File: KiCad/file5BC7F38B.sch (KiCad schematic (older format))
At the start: 54 parts, among them J307 Jumper_NC_Small, P301 ISP/PDI, P302 Thru, P303 Header, P304 Header, U301 DS3231, U302 TS5A3157, U303 ATMEGA328P, U304 SI5351A, U305 74HC1G08, U306 MIC5219-3.3BM5, U307 SN74CB3Q3305, U308 MIC5219-3.3BM5, X301 ASTX-H11-25.MHZ

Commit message: Changes for FlexFox80
Wholesale changes for new project.
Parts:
- removed C303: 100nF, Capacitors_SMD:C_0805_HandSoldering, symbol Device:C_Small
- removed U302: TS5A3157, TO_SOT_Packages_SMD:SOT-363_Handsolder, symbol ARDF-2-Band-MiniTx-rescue:TS5A3159
- added U?: ATmega1284P-AU, Package_QFP:TQFP-44_10x10mm_P0.8mm, symbol MCU_Microchip_ATmega:ATmega1284P-AU
- BT301: symbol ARDF-2-Band-MiniTx-rescue:Battery_Single_Cell -> FlexFox80-rescue:Battery_Single_Cell-ARDF-2-Band-MiniTx-rescue
- D301: symbol ARDF-2-Band-MiniTx-rescue:D_Schottky_x2_KCom_Dual -> FlexFox80-rescue:D_Schottky_x2_KCom_Dual-ARDF-2-Band-MiniTx-rescue
- D302: symbol ARDF-2-Band-MiniTx-rescue:ZENER -> FlexFox80-rescue:ZENER-ARDF-2-Band-MiniTx-rescue
- D303: symbol ARDF-2-Band-MiniTx-rescue:MBD54DWT1G_Schottky_Ind -> FlexFox80-rescue:MBD54DWT1G_Schottky_Ind-ARDF-2-Band-MiniTx-rescue
- P301: symbol ARDF-2-Band-MiniTx-rescue:CONN_02X03 -> FlexFox80-rescue:CONN_02X03-ARDF-2-Band-MiniTx-rescue
- P302, W307, W308: symbol ARDF-2-Band-MiniTx-rescue:CONN_01X01 -> FlexFox80-rescue:CONN_01X01-ARDF-2-Band-MiniTx-rescue
- P303, P304: symbol ARDF-2-Band-MiniTx-rescue:CONN_01X06 -> FlexFox80-rescue:CONN_01X06-ARDF-2-Band-MiniTx-rescue
- TP301: symbol ARDF-2-Band-MiniTx-rescue:CONN_01X03 -> FlexFox80-rescue:CONN_01X03-ARDF-2-Band-MiniTx-rescue
- U303: symbol ARDF-2-Band-MiniTx-rescue:ATMEGA328P-A -> FlexFox80-rescue:ATMEGA328P-A-ARDF-2-Band-MiniTx-rescue
- U305: symbol ARDF-2-Band-MiniTx-rescue:74HC1G08 -> FlexFox80-rescue:74HC1G08-ARDF-2-Band-MiniTx-rescue
- U306, U308: symbol ARDF-2-Band-MiniTx-rescue:MIC5219 -> FlexFox80-rescue:MIC5219-ARDF-2-Band-MiniTx-rescue
- U307: symbol ARDF-2-Band-MiniTx-rescue:SN74CB3Q3305 -> FlexFox80-rescue:SN74CB3Q3305-ARDF-2-Band-MiniTx-rescue
- W301, W302, W309, W310, W311, W312, W313, W314, W315, W316: symbol ARDF-2-Band-MiniTx-rescue:TEST_1P -> FlexFox80-rescue:TEST_1P-ARDF-2-Band-MiniTx-rescue
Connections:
- net labels removed: VHF_CLK
- wire segments 189 -> 245
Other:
- note added: "PCB: Flex Fox 80 ARDF Transmitter (p. 3/3)"
- note removed: "PCB: Dual-Band Transmitter (p. 3/3)"

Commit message: Schematic
Schematic changes for FlexFox80
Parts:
- removed U303: ATMEGA328P, Housings_QFP:TQFP-32_7x7mm_Pitch0.8mm, symbol FlexFox80-rescue:ATMEGA328P-A-ARDF-2-Band-MiniTx-rescue
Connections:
- net labels added: ADC3, ADC4, HT_AUDIO_IN, INT2, PC4, PC5, RXD0, RXD1, TXD0, TXD1
- net labels removed: 2M_ANTENNA_DETECT, PD2, VHF_ENABLE
- wire segments 245 -> 263
- no-connect marks 12 -> 24
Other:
- moved on the sheet: BT301, C301, C302, C304, C305, C306, C307, C308, C310, C312, C314, C316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

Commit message: Schematic Updates
More schematic changes
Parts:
- removed J307: Jumper_NC_Small, Wire_Connections_Bridges:Solder-Jumper-NC-SMD-Pad_Small, symbol Device:Jumper_NC_Small
- added Y301: 20 MHz, symbol Device:Resonator_Small
- gave numbers to parts that had none: 1
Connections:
- net labels added: KEY_OUT, PA0, PA1, PA2, PA3, PC6, PC7, PTT_OUT, TONE_OUT
- net labels removed: PB2, PB6, PB7, PC0, PC1, PD0, PD1, PD3, VHF_CLK_SEL
- wire segments 263 -> 258
- no-connect marks 24 -> 17
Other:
- moved on the sheet: C309, D303A, P303, R304, R305

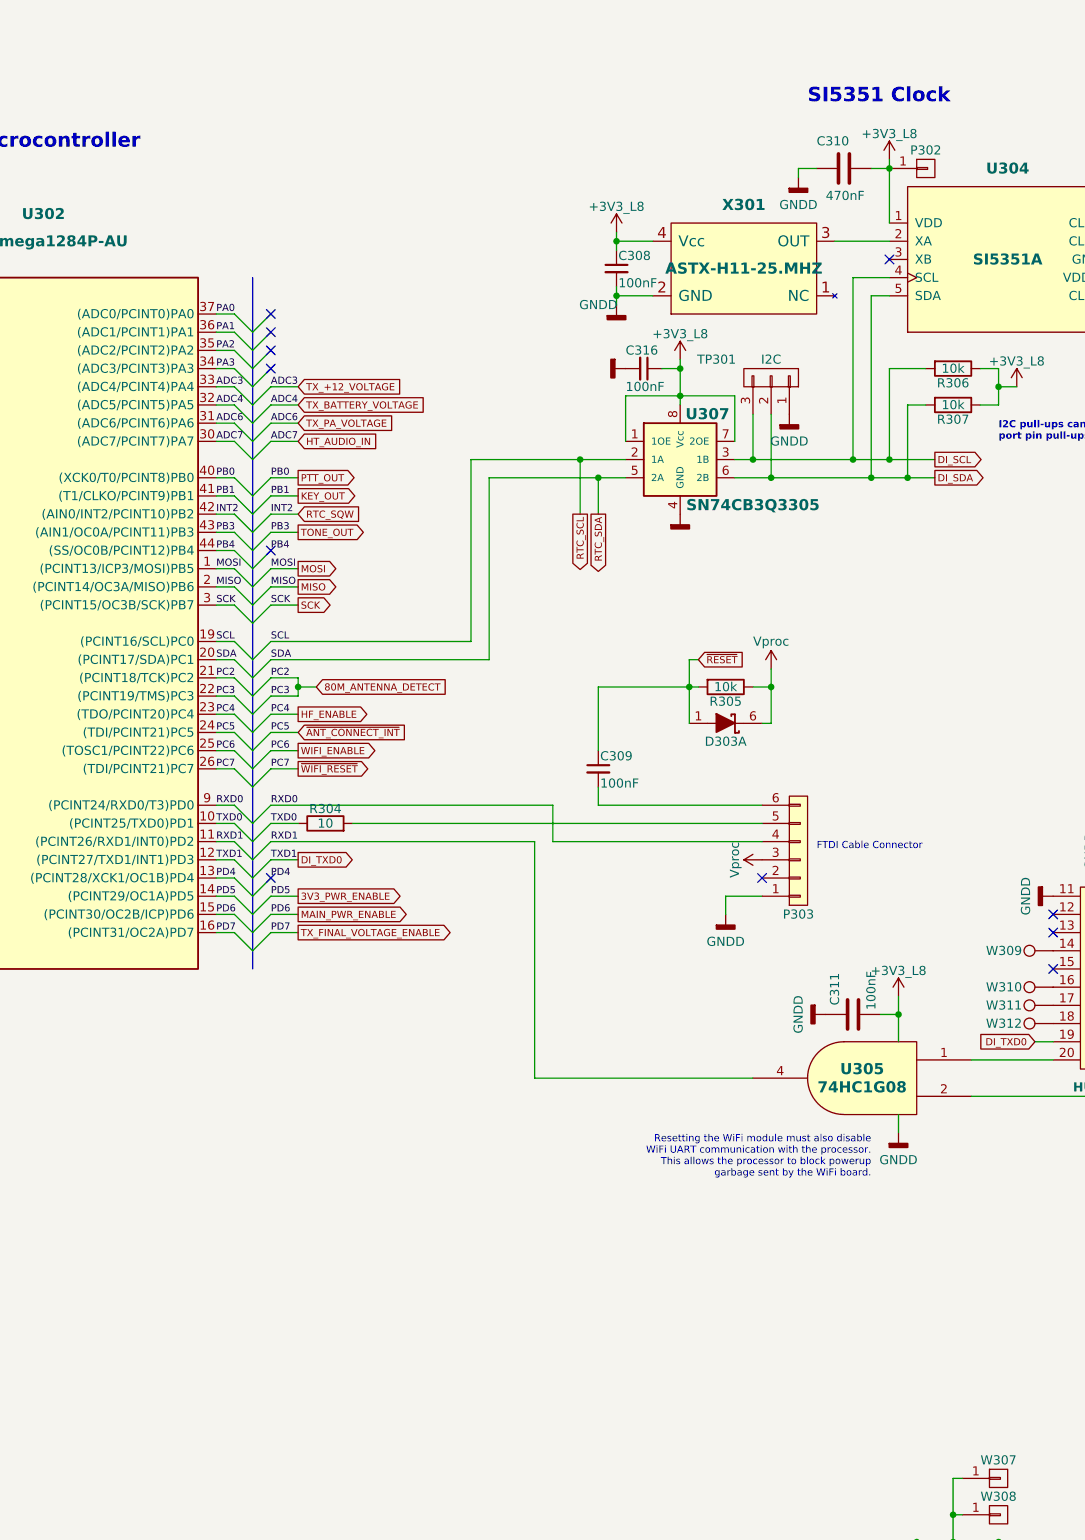
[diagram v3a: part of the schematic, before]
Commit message: Schematic changes
Schematic
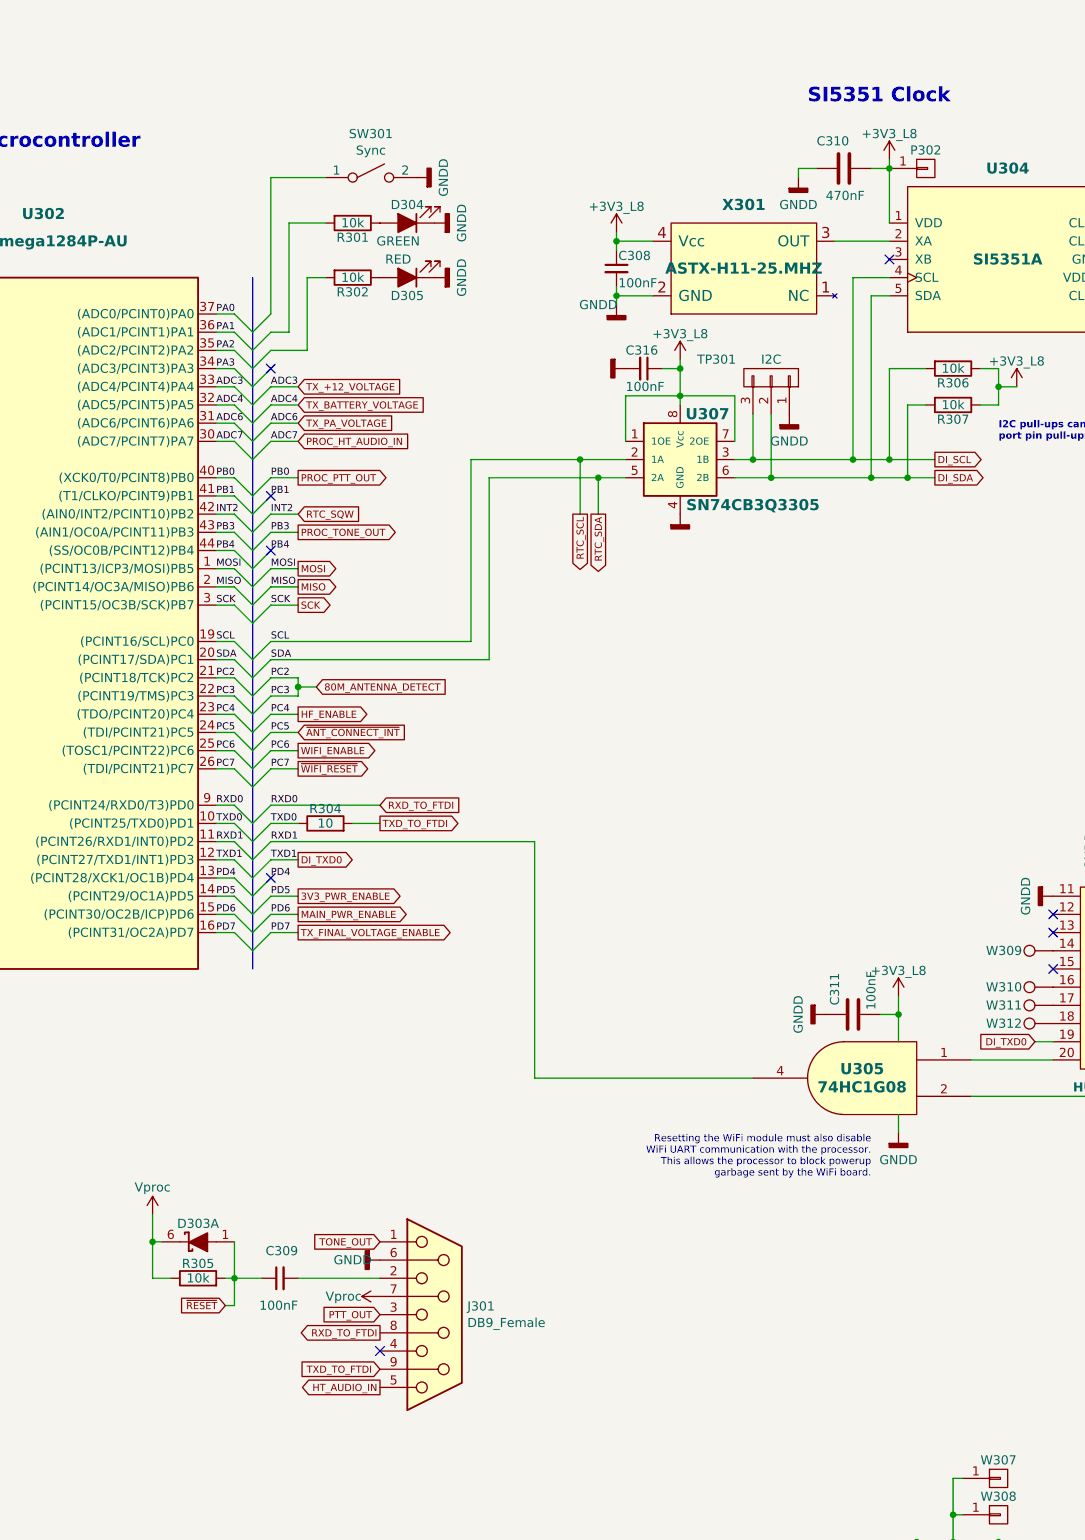
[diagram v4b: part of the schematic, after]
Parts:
- removed P303: Header, Pin_Headers:Pin_Header_Straight_1x06, symbol FlexFox80-rescue:CONN_01X06-ARDF-2-Band-MiniTx-rescue
- added D304: GREEN, symbol Device:LED_ALT
- added D305: RED, symbol Device:LED_ALT
- added J301: DB9_Female, symbol Connector:DB9_Female
- added R301, R302: 10k, Resistors_SMD:R_0805_HandSoldering, symbol Device:R
- added SW301: Sync, symbol Switch:SPST_small
- Y301: Part No. (none) -> CSTNE20M0V53Z000R0
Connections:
- net GND: now also D304.1 (K), D305.1 (K), J301.6, SW301.2
- net HT_AUDIO_IN: now also J301.5; no longer U302.30 ((ADC7/PCINT7)PA7)
- net PTT_OUT: now also J301.3; no longer U302.40 ((XCK0/T0/PCINT8)PB0)
- net Vproc: now also J301.7
- net TXD_TO_FTDI: now reaches R304.2
- net TXD_TO_FTDI: now also J301.9
- net at C309.2: now also J301.2
- net KEY_OUT renamed PB1
- net RXD0 renamed RXD_TO_FTDI
- net RXD_TO_FTDI: now also J301.8
- new net: D304.2 (A), R301.1
- new net: D305.2 (A), R302.1
- new net PROC_HT_AUDIO_IN: U302.30 ((ADC7/PCINT7)PA7)
- new net PROC_PTT_OUT: U302.40 ((XCK0/T0/PCINT8)PB0)
- new net TONE_OUT: J301.1
- no-connect marks 17 -> 15
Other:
- moved on the sheet: C309, D303A, R305
